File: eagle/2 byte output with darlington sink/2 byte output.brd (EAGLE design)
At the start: 82.5 x 50.5 mm, 13 parts, among them IC1 74LS595N, IC2 74LS595N, X1 MKDSN1,5/8-5,08, X2 MKDSN1,5/8-5,08, X3 MKDSN1,5/5-5,08, X4 MKDSN1,5/5-5,08, X5 MKDSN1,5/2-5,08

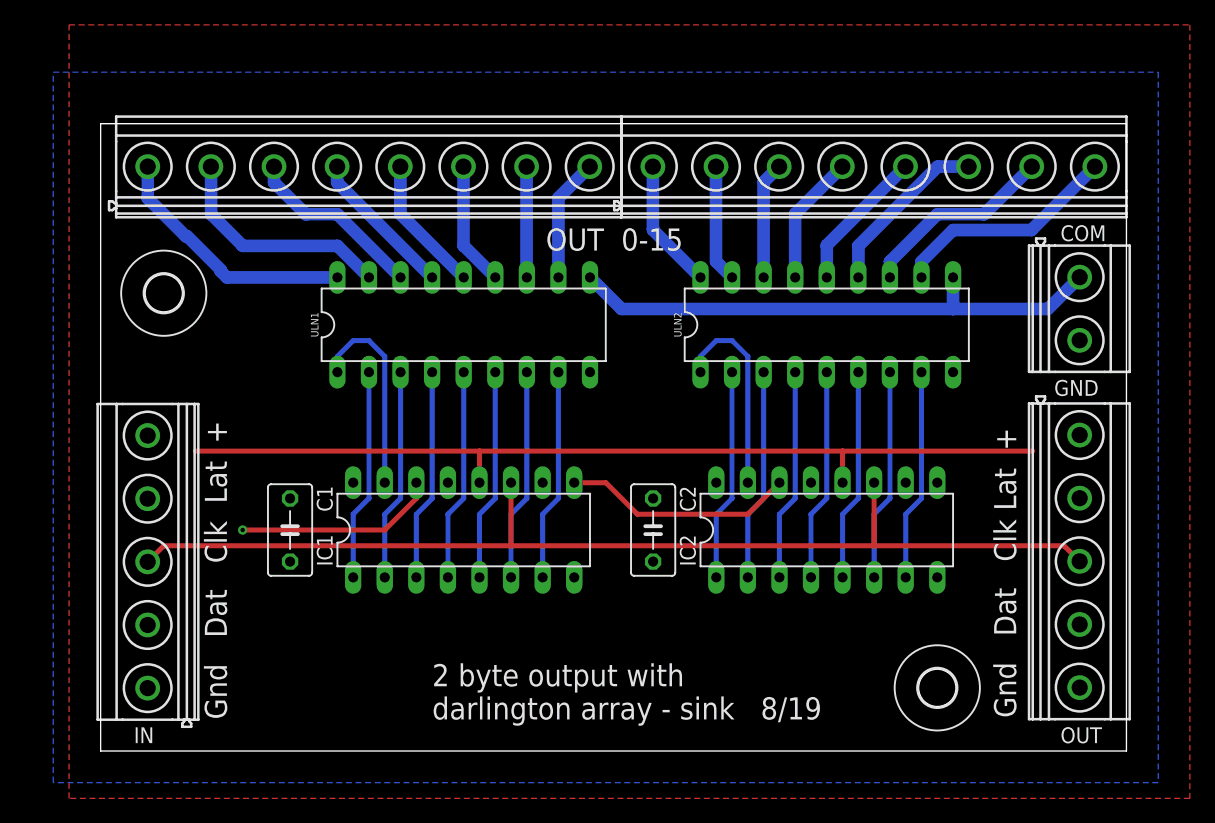
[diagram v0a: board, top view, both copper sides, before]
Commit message: periodic check-in
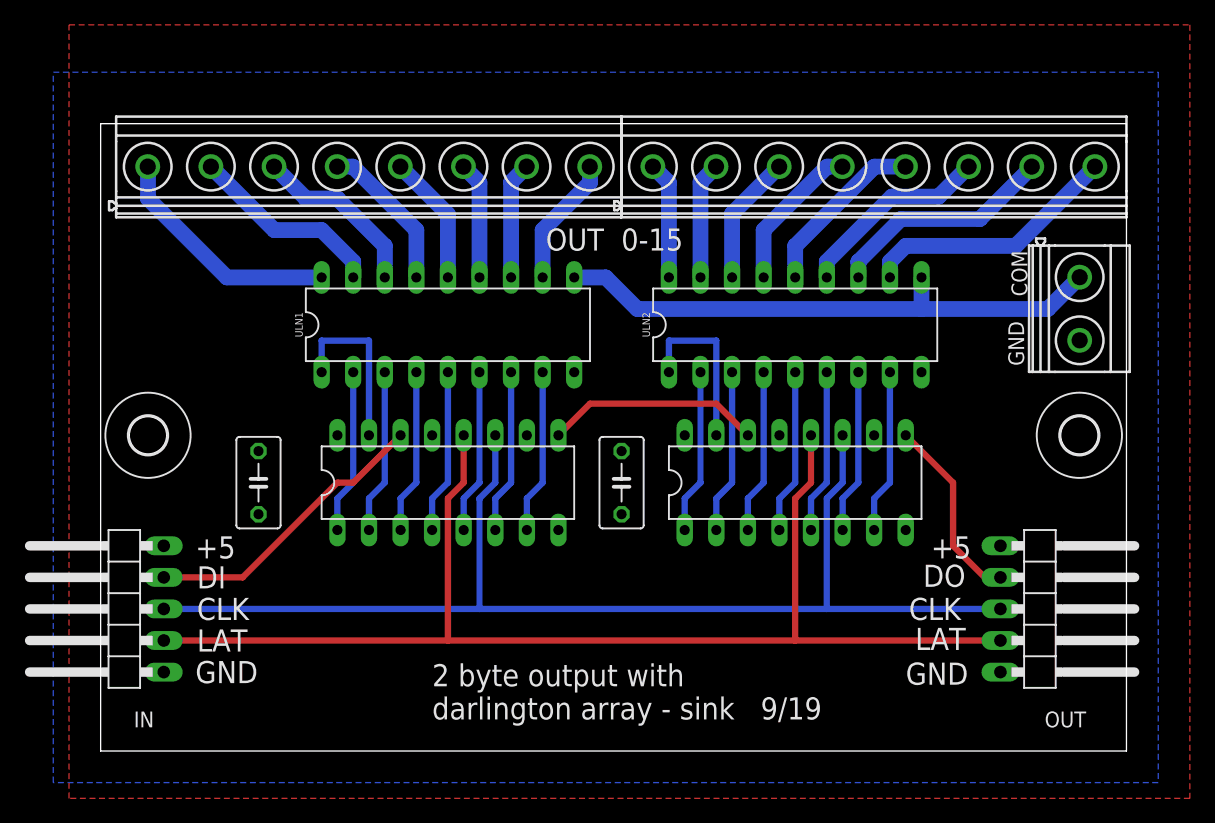
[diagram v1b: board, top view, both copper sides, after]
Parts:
- removed X3, X4: MKDSN1,5/5-5,08, con-phoenix-508:MKDSN1,5/5-5,08
- added JP1, JP2: (no value), pinhead:1X05/90
- ULN1: value (none) -> ULN2803
- ULN2: value (none) -> uln2803
- moved H2 23.3 mm to (78.7, 25.4)
- moved H1 11.5 mm to (3.81, 25.4)
- moved C2 4.58 mm to (41.9, 21.6)
- moved C1 4.58 mm to (12.7, 21.6)
- moved IC2 4.58 mm to (55.9, 21.6)
- moved IC1 4.02 mm to (27.9, 21.6)
- moved ULN2 2.54 mm to (55.9, 34.3)
- moved ULN1 1.27 mm to (27.9, 34.3)
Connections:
- net CLK: now also JP1.3, JP2.3; no longer X3.3, X4.3
- net DI: now also JP2.4; no longer X3.4
- net DO: now also JP1.2; no longer X4.2
- net GND: now also JP1.5, JP2.1; no longer X3.1, X4.5
- net LATCH: now also JP1.4, JP2.2; no longer X3.2, X4.4
- net VCC: now also JP1.1, JP2.5; no longer X3.5, X4.1
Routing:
- net LATCH: track 72.4 -> 101.4 mm
- net DO: track 0.05 -> 15.3 mm
- net CLK: track 86.2 -> 96.3 mm
- net DI: track 16.3 -> 23.8 mm, vias 1 -> 0
- net OUT15: track 17.0 -> 13.2 mm
- net OUT10: track 17.0 -> 13.2 mm
- net OUT3: track 17.0 -> 13.2 mm
- net OUT9: track 17.0 -> 13.2 mm
- net OUT5: track 17.0 -> 13.2 mm
- net OUT4: track 17.0 -> 13.2 mm
- net OUT2: track 17.0 -> 13.2 mm
- net OUT14: track 17.0 -> 13.2 mm
- net OUT13: track 17.0 -> 13.2 mm
- net OUT12: track 17.0 -> 13.2 mm
- net OUT11: track 17.0 -> 13.2 mm
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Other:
- board text added: "+5"
- board text added: "2 byte output with darlington array - sink 9/19"
- board text added: "CLK"
- board text added: "DI"
- board text added: "DO"
- board text added: "LAT"
- board text removed: "2 byte output with darlington array - sink 8/19"
- board text removed: "Gnd Dat Clk Lat +"
